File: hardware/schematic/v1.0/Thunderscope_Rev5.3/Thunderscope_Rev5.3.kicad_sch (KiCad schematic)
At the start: 16 parts

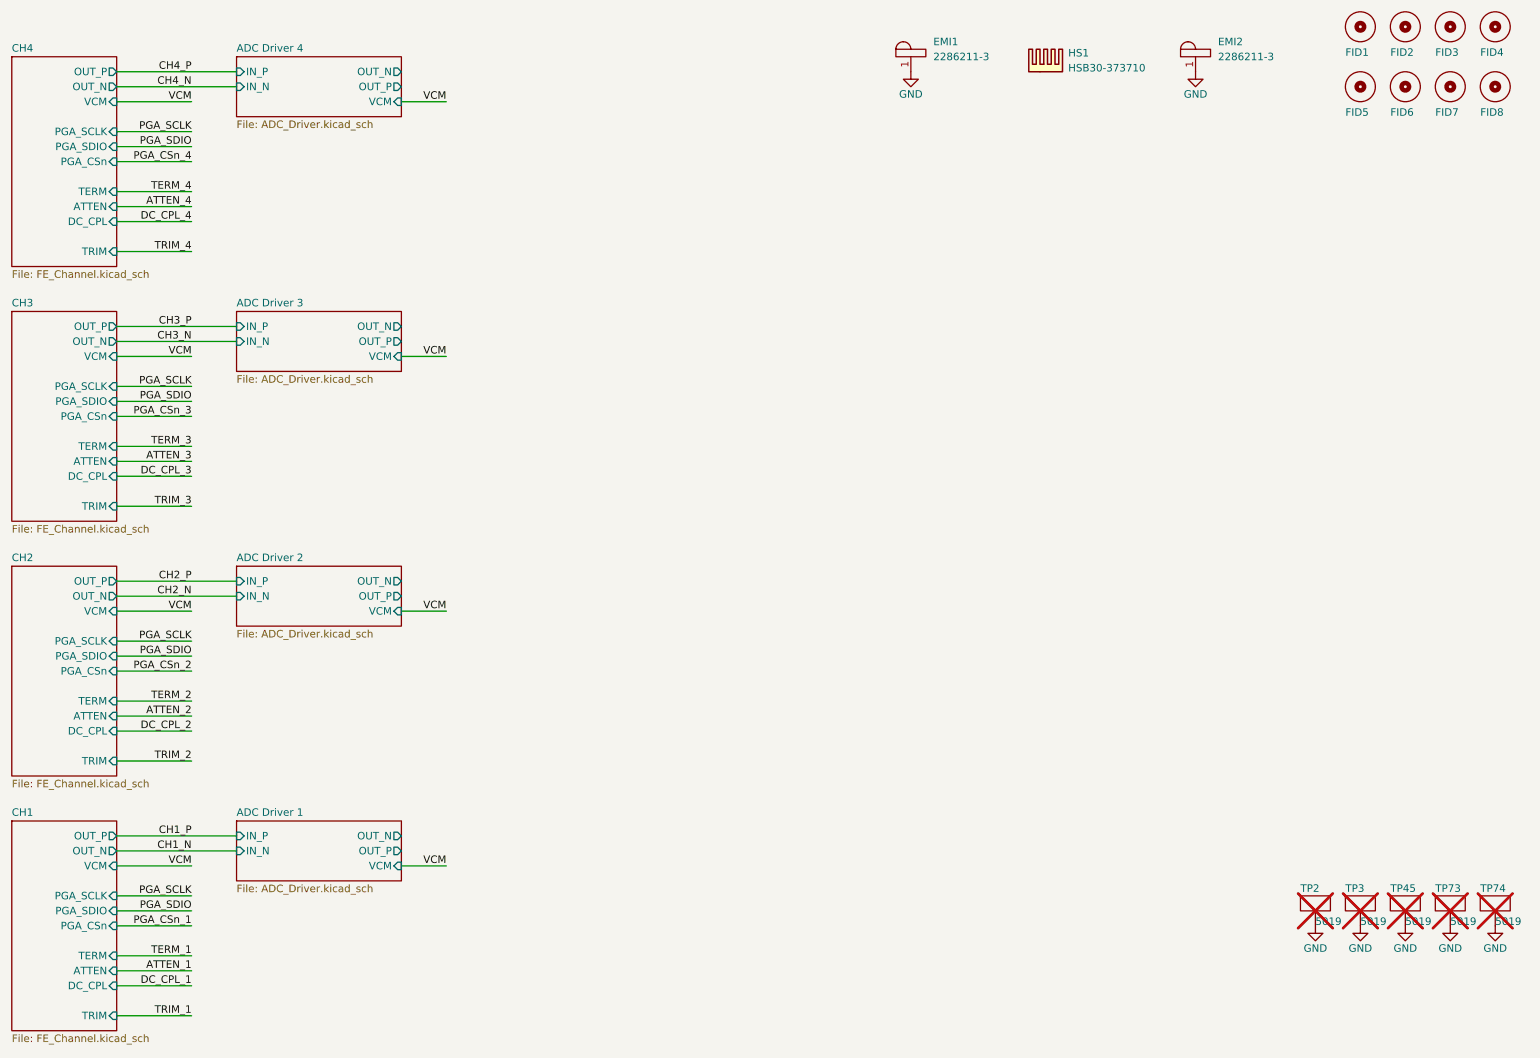
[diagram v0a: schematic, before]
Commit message: sch update
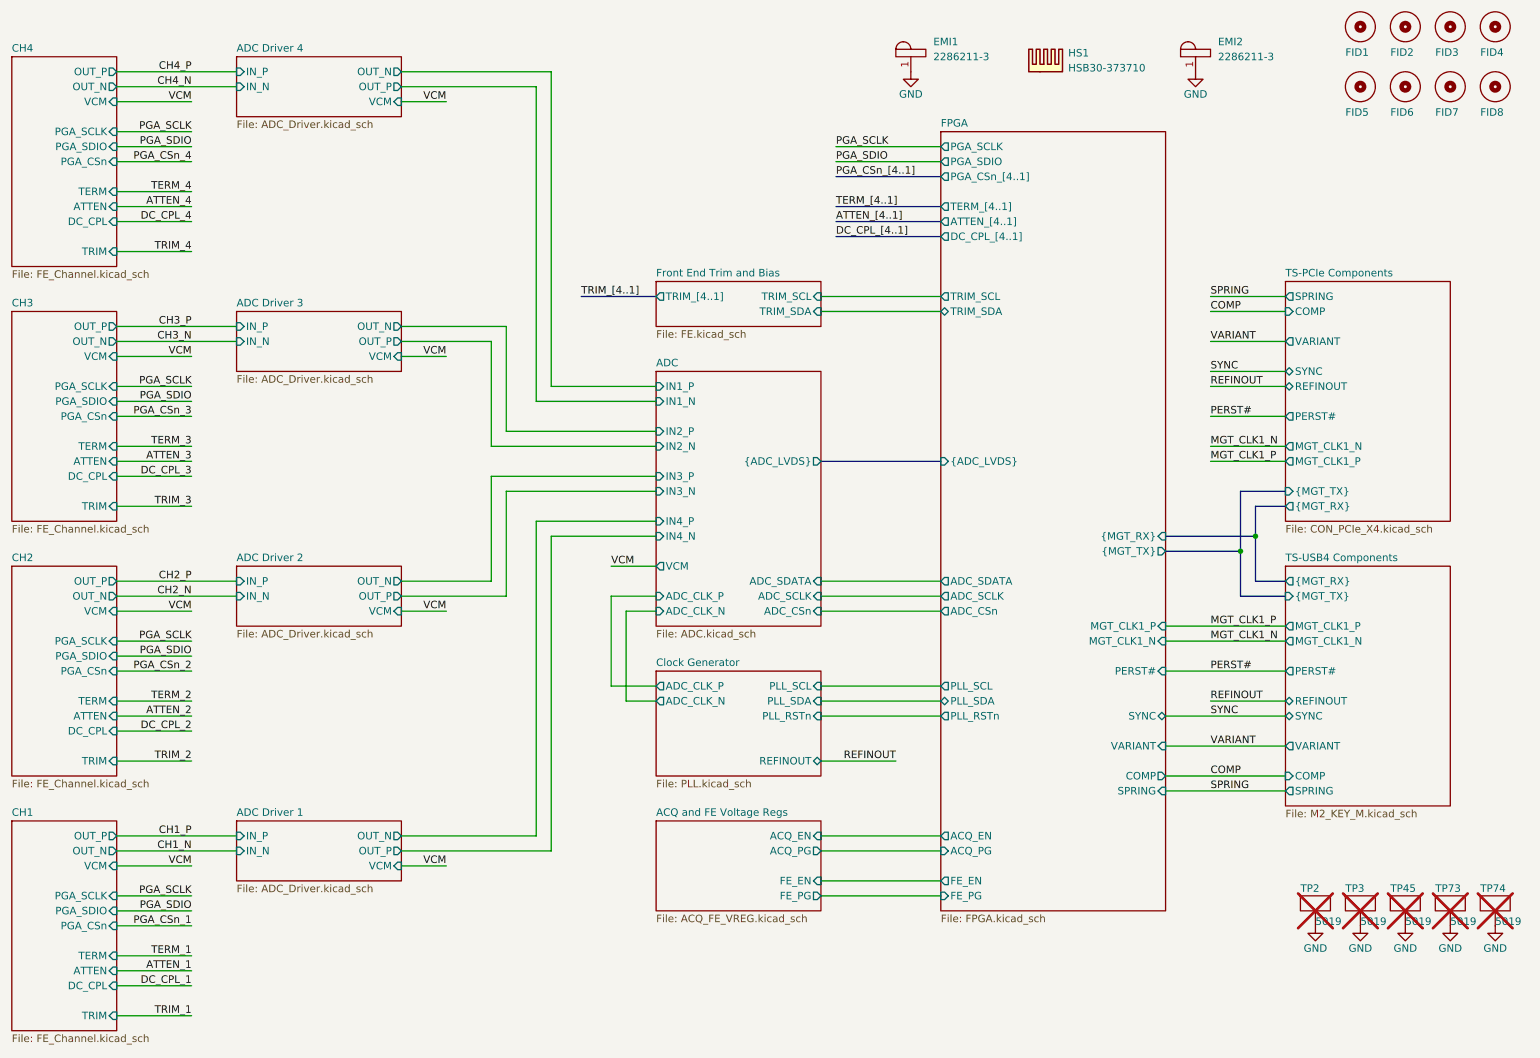
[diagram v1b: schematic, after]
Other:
- added sheet ACQ and FE Voltage Regs (ACQ_FE_VREG.kicad_sch)
- added sheet ADC (ADC.kicad_sch)
- added sheet Clock Generator (PLL.kicad_sch)
- added sheet FPGA (FPGA.kicad_sch)
- added sheet Front End Trim and Bias (FE.kicad_sch)
- added sheet TS-PCIe Components (CON_PCIe_X4.kicad_sch)
- added sheet TS-USB4 Components (M2_KEY_M.kicad_sch)
